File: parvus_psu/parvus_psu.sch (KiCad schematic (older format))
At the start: 67 parts, among them J1 tr_sec, J2 switch, J3 ac_input, J4 tr_pri, J5 power_1, J6 power_2, J7 signal, J8 ctrl_1, J9 ctrl_2, Q1 BC546B, Q2 BC546B, Q3 BC546B, Q4 BC546B, Q5 BC546B, Q6 BC556B, Q7 BC556B, Q8 BC556B

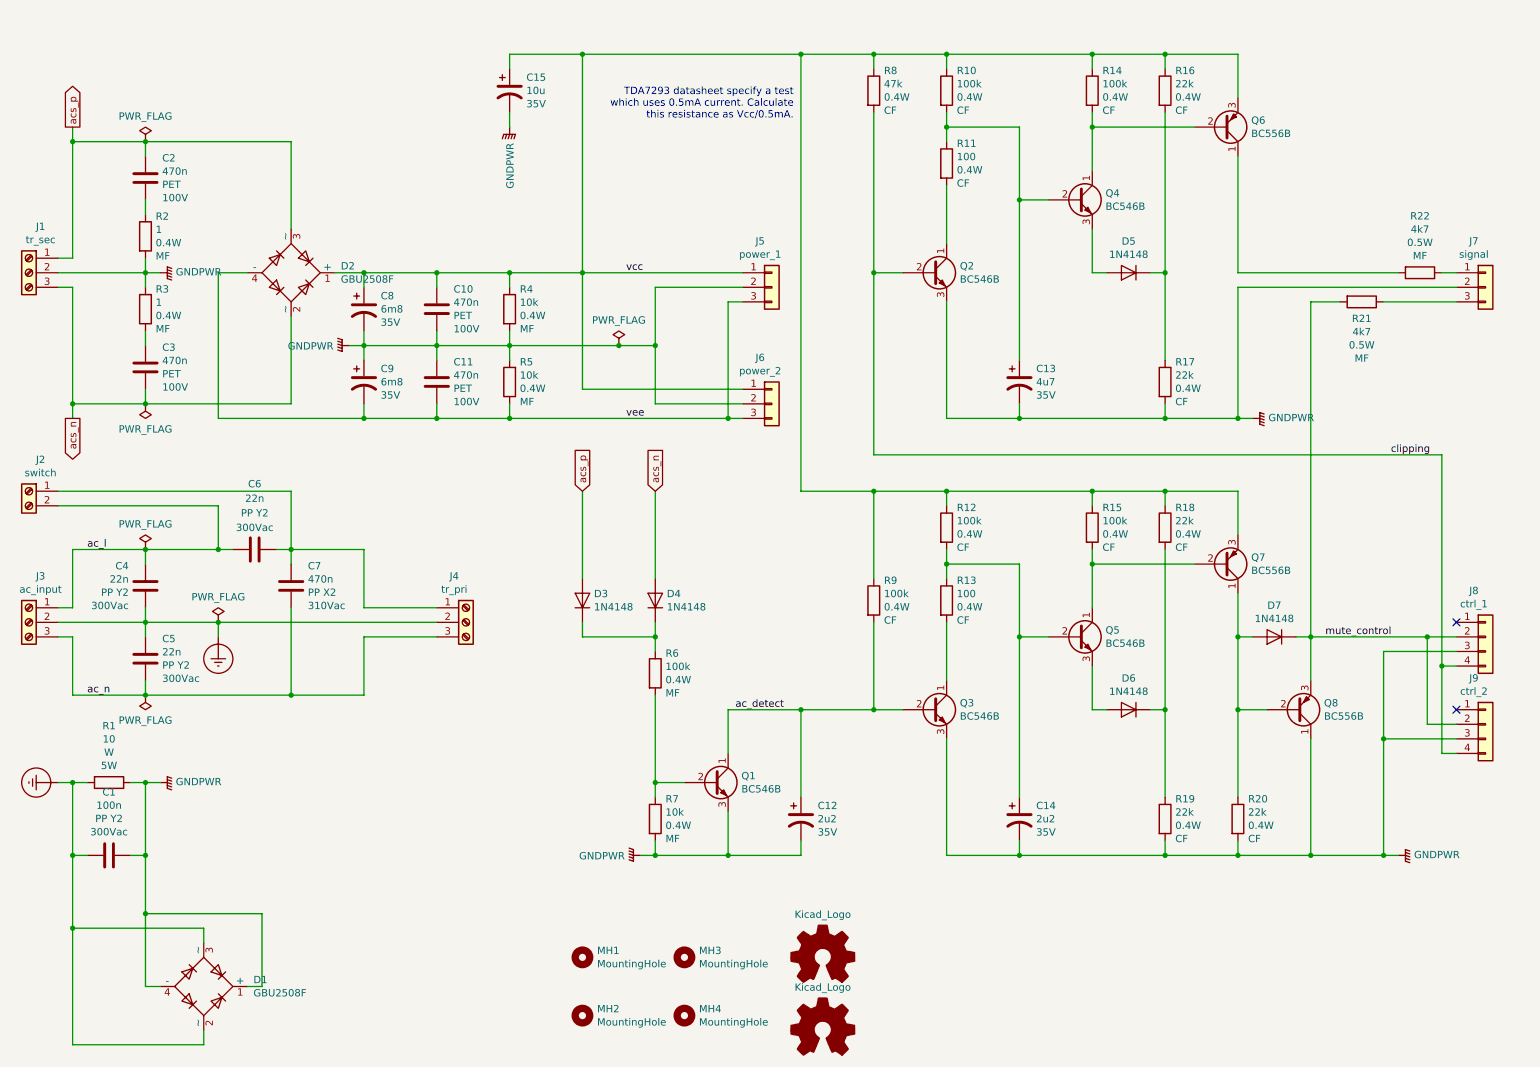
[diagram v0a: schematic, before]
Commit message: Updated to new version v1.02.
Signed-off-by: Nenad Radulovic <nenad.b.radulovic@gmail.com>
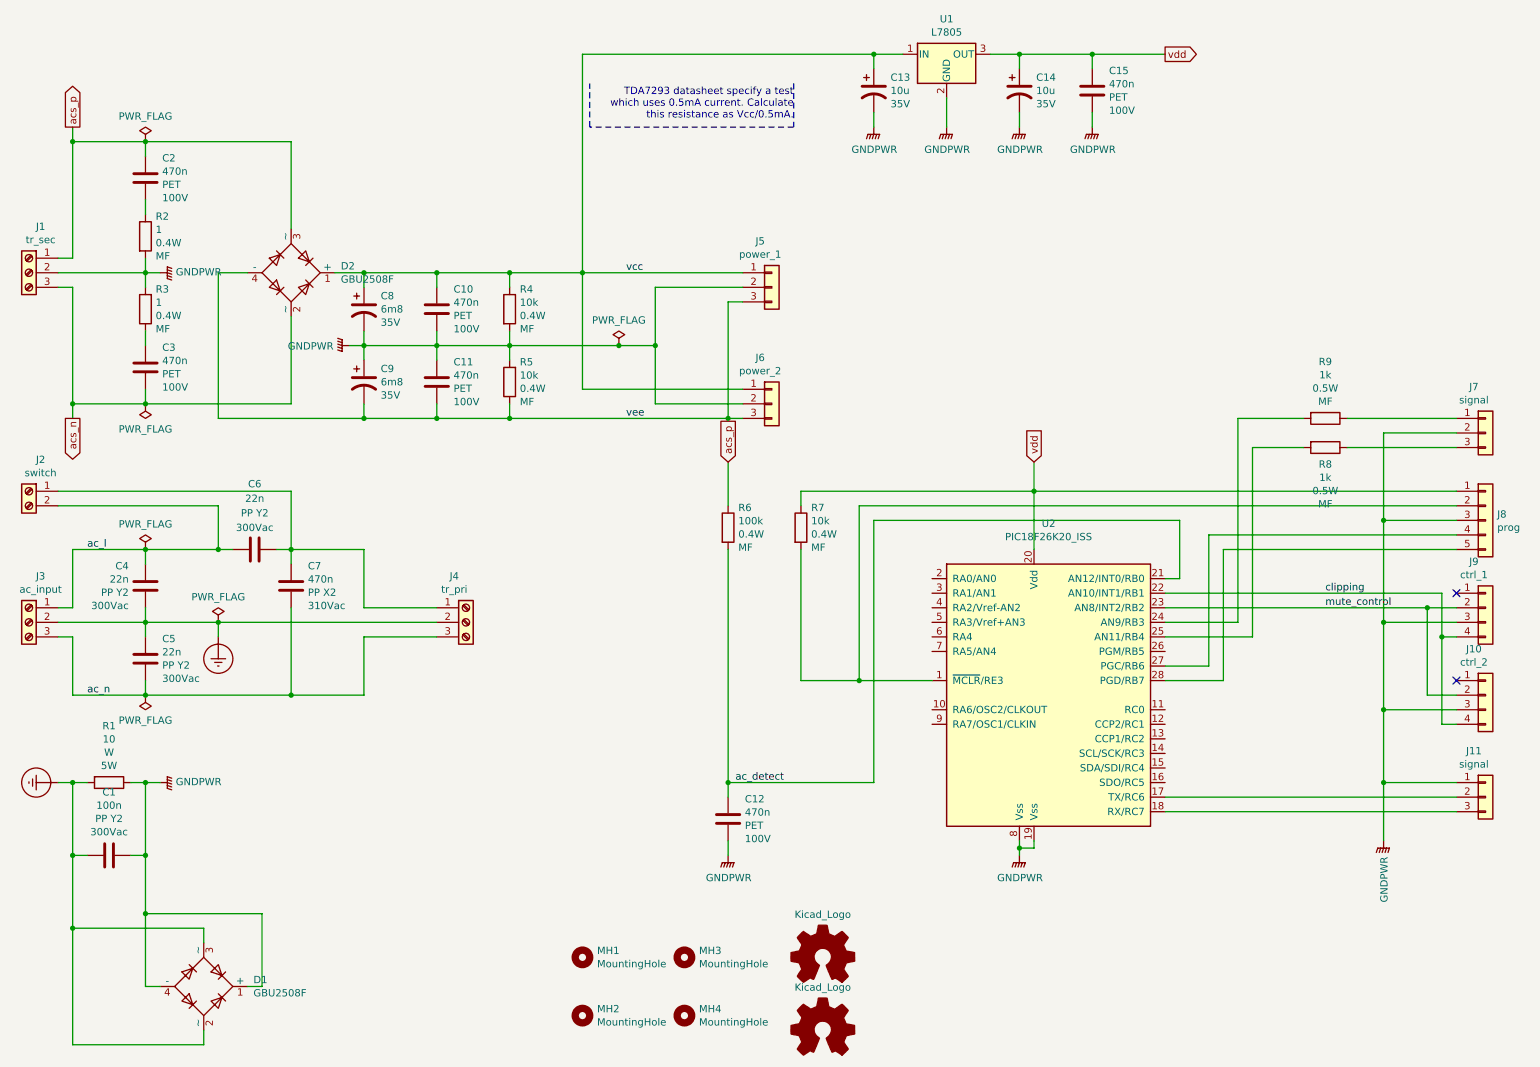
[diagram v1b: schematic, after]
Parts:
- removed C12: 2u2, Capacitor_THT:CP_Radial_D5.0mm_P2.50mm, symbol Device:CP1
- removed C13: 4u7, Capacitor_THT:CP_Radial_D5.0mm_P2.50mm, symbol Device:CP1
- removed D3, D4, D5, D6, D7: 1N4148, Diode_THT:D_DO-35_SOD27_P7.62mm_Horizontal, symbol Device:D
- removed Q1, Q2, Q3, Q4, Q5: BC546B, Package_TO_SOT_THT:TO-92_Inline_Wide, symbol Device:Q_NPN_CBE
- removed Q6, Q7, Q8: BC556B, Package_TO_SOT_THT:TO-92_Inline_Wide, symbol Device:Q_PNP_CBE
- removed R10, R12, R14, R15, R9: 100k, Resistor_THT:R_Axial_DIN0207_L6.3mm_D2.5mm_P10.16mm_Horizontal, symbol Device:R
- removed R11, R13: 100, Resistor_THT:R_Axial_DIN0207_L6.3mm_D2.5mm_P10.16mm_Horizontal, symbol Device:R
- removed R16, R17, R18, R19, R20: 22k, Resistor_THT:R_Axial_DIN0207_L6.3mm_D2.5mm_P10.16mm_Horizontal, symbol Device:R
- removed R8: 47k, Resistor_THT:R_Axial_DIN0207_L6.3mm_D2.5mm_P10.16mm_Horizontal, symbol Device:R
- added C12, C15: 470n, Capacitor_THT:C_Rect_L7.2mm_W8.5mm_P5.00mm_FKP2_FKP2_MKS2_MKP2, symbol Device:C
- added J11: signal, Connector_PinHeader_2.54mm:PinHeader_1x03_P2.54mm_Vertical, symbol Connector_Generic:Conn_01x03
- added J8: prog, Connector_PinHeader_2.54mm:PinHeader_1x04_P2.54mm_Vertical, symbol Connector_Generic:Conn_01x05
- added U1: L7805, Package_TO_SOT_THT:TO-220-3_Vertical, symbol Regulator_Linear:L7805
- added U2: PIC18F26K20_ISS, Package_DIP:DIP-28_W7.62mm_LongPads, symbol MCU_Microchip_PIC18:PIC18F26K20_ISS
- C14: value 2u2 -> 10u; footprint Capacitor_THT:CP_Radial_D5.0mm_P2.50mm -> Capacitor_THT:CP_Radial_D8.0mm_P2.50mm
- R8: renamed from R21; value 4k7 -> 1k; footprint Resistor_THT:R_Axial_DIN0309_L9.0mm_D3.2mm_P12.70mm_Horizontal -> Resistor_THT:R_Axial_DIN0207_L6.3mm_D2.5mm_P10.16mm_Horizontal
- R9: renamed from R22; value 4k7 -> 1k; footprint Resistor_THT:R_Axial_DIN0309_L9.0mm_D3.2mm_P12.70mm_Horizontal -> Resistor_THT:R_Axial_DIN0207_L6.3mm_D2.5mm_P10.16mm_Horizontal
- renumbered C15 to C13, J9 to J10, J8 to J9
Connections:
- net GNDPWR: now also C12.2, C15.2, J11.1 (Pin_1), J8.3 (Pin_3), U1.2 (GND), U2.19 (Vss), U2.8 (Vss); no longer R7.2
- net ac_detect: now also R6.2, C12.1, U2.21 (AN12/INT0/RB0)
- net acs_p: now also R6.1
- net clipping: now also U2.22 (AN10/INT1/RB1)
- net mute_control: now also U2.23 (AN8/INT2/RB2); no longer R8.2
- net vcc: now also U1.1 (IN)
- net vdd: now reaches R7.1
- net vdd: now also C14.1, C15.1, J8.1 (Pin_1), U1.3 (OUT), U2.20 (Vdd); no longer R6.2
- net at R9.2: now also U2.24 (AN9/RB3)
- new net: R8.2, U2.25 (AN11/RB4)
- new net: J8.2 (Pin_2), R7.2, U2.1 (~MCLR~/RE3)
- new net: J11.2 (Pin_2), U2.17 (TX/RC6)
- new net: J11.3 (Pin_3), U2.18 (RX/RC7)
- new net: J8.4 (Pin_4), U2.27 (PGC/RB6)
- new net: J8.5 (Pin_5), U2.28 (PGD/RB7)
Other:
- moved on the sheet: C13, J10, J7, J9, R6, R8, R9

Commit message: Project update
Signed-off-by: Nenad Radulovic <nenad.b.radulovic@gmail.com>
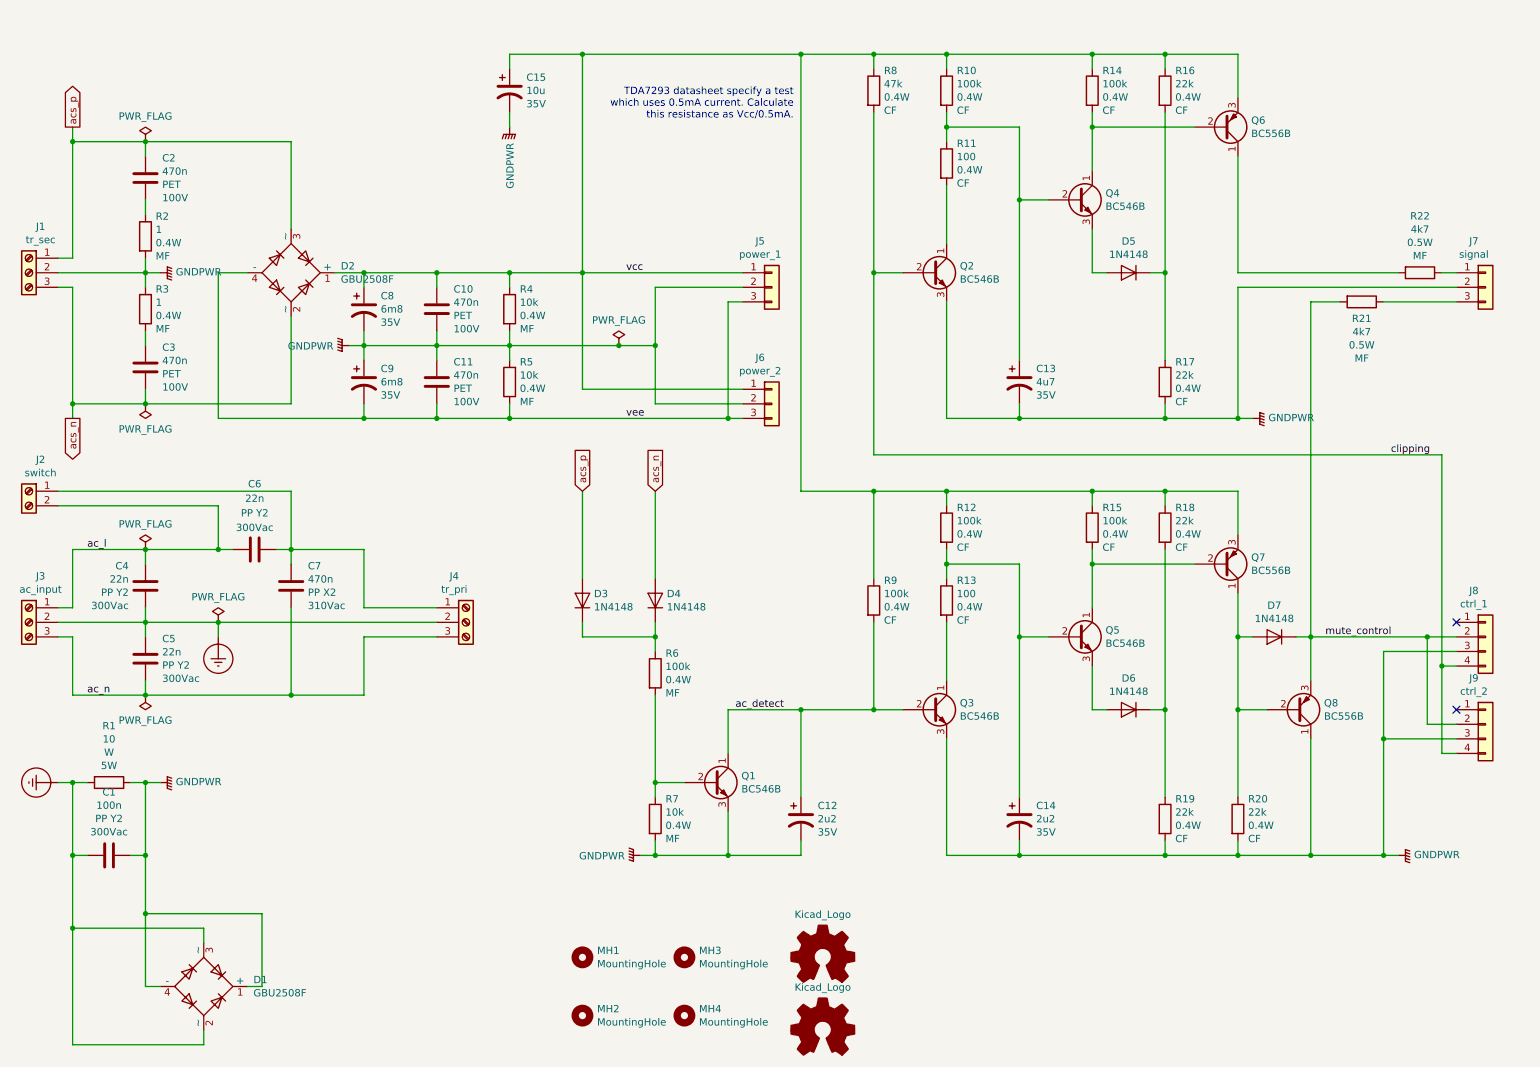
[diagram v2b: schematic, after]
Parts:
- removed C12, C15: 470n, Capacitor_THT:C_Rect_L7.2mm_W8.5mm_P5.00mm_FKP2_FKP2_MKS2_MKP2, symbol Device:C
- removed J11: signal, Connector_PinHeader_2.54mm:PinHeader_1x03_P2.54mm_Vertical, symbol Connector_Generic:Conn_01x03
- removed J8: prog, Connector_PinHeader_2.54mm:PinHeader_1x04_P2.54mm_Vertical, symbol Connector_Generic:Conn_01x05
- removed U1: L7805, Package_TO_SOT_THT:TO-220-3_Vertical, symbol Regulator_Linear:L7805
- removed U2: PIC18F26K20_ISS, Package_DIP:DIP-28_W7.62mm_LongPads, symbol MCU_Microchip_PIC18:PIC18F26K20_ISS
- added C12: 2u2, Capacitor_THT:CP_Radial_D5.0mm_P2.50mm, symbol Device:CP1
- added C13: 4u7, Capacitor_THT:CP_Radial_D5.0mm_P2.50mm, symbol Device:CP1
- added D3, D4, D5, D6, D7: 1N4148, Diode_THT:D_DO-35_SOD27_P7.62mm_Horizontal, symbol Device:D
- added Q1, Q2, Q3, Q4, Q5: BC546B, Package_TO_SOT_THT:TO-92_Inline_Wide, symbol Device:Q_NPN_CBE
- added Q6, Q7, Q8: BC556B, Package_TO_SOT_THT:TO-92_Inline_Wide, symbol Device:Q_PNP_CBE
- added R10, R12, R14, R15, R9: 100k, Resistor_THT:R_Axial_DIN0207_L6.3mm_D2.5mm_P10.16mm_Horizontal, symbol Device:R
- added R11, R13: 100, Resistor_THT:R_Axial_DIN0207_L6.3mm_D2.5mm_P10.16mm_Horizontal, symbol Device:R
- added R16, R17, R18, R19, R20: 22k, Resistor_THT:R_Axial_DIN0207_L6.3mm_D2.5mm_P10.16mm_Horizontal, symbol Device:R
- added R8: 47k, Resistor_THT:R_Axial_DIN0207_L6.3mm_D2.5mm_P10.16mm_Horizontal, symbol Device:R
- C14: value 10u -> 2u2; footprint Capacitor_THT:CP_Radial_D8.0mm_P2.50mm -> Capacitor_THT:CP_Radial_D5.0mm_P2.50mm
- R21: renamed from R8; value 1k -> 4k7; footprint Resistor_THT:R_Axial_DIN0207_L6.3mm_D2.5mm_P10.16mm_Horizontal -> Resistor_THT:R_Axial_DIN0309_L9.0mm_D3.2mm_P12.70mm_Horizontal
- R22: renamed from R9; value 1k -> 4k7; footprint Resistor_THT:R_Axial_DIN0207_L6.3mm_D2.5mm_P10.16mm_Horizontal -> Resistor_THT:R_Axial_DIN0309_L9.0mm_D3.2mm_P12.70mm_Horizontal
- renumbered C13 to C15, J9 to J8, J10 to J9
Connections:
- net GNDPWR: now also R7.2, C12.2, C13.2, Q1.3 (E), Q2.3 (E), Q3.3 (E), Q8.1 (C), R17.2, R19.2, R20.2
- net ac_detect: now also C12.1, Q1.1 (C), Q3.2 (B), R9.2; no longer R6.2
- net acs_n: now also D4.2 (A)
- net acs_p: now also D3.2 (A); no longer R6.1
- net clipping: now also Q2.2 (B), R8.2
- net mute_control: now also R21.2, D7.1 (K), Q8.3 (E)
- net vcc: now also Q6.3 (E), Q7.3 (E), R10.1, R12.1, R14.1, R15.1, R16.1, R18.1, R8.1, R9.1
- net at R22.2: now also Q6.1 (C)
- net vdd: no longer names the net of R7.1
- net vdd: now also R6.2, Q1.2 (B); no longer C14.1
- new net: D3.1 (K), D4.1 (K), R6.1
- new net: Q3.1 (C), R13.2
- new net: C14.1, Q5.2 (B), R12.2, R13.1
- new net: D7.2 (A), Q7.1 (C), Q8.2 (B), R20.1
- new net: Q5.1 (C), Q7.2 (B), R15.2
- new net: D6.1 (K), R18.2, R19.1
- new net: D6.2 (A), Q5.3 (E)
- new net: Q2.1 (C), R11.2
- new net: C13.1, Q4.2 (B), R10.2, R11.1
- new net: Q4.1 (C), Q6.2 (B), R14.2
- new net: D5.1 (K), R16.2, R17.1
- new net: D5.2 (A), Q4.3 (E)
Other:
- moved on the sheet: C15, J7, J8, J9, R21, R22, R6
